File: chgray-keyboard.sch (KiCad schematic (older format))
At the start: 1 part, among them U1 Teensy2.0_(C)

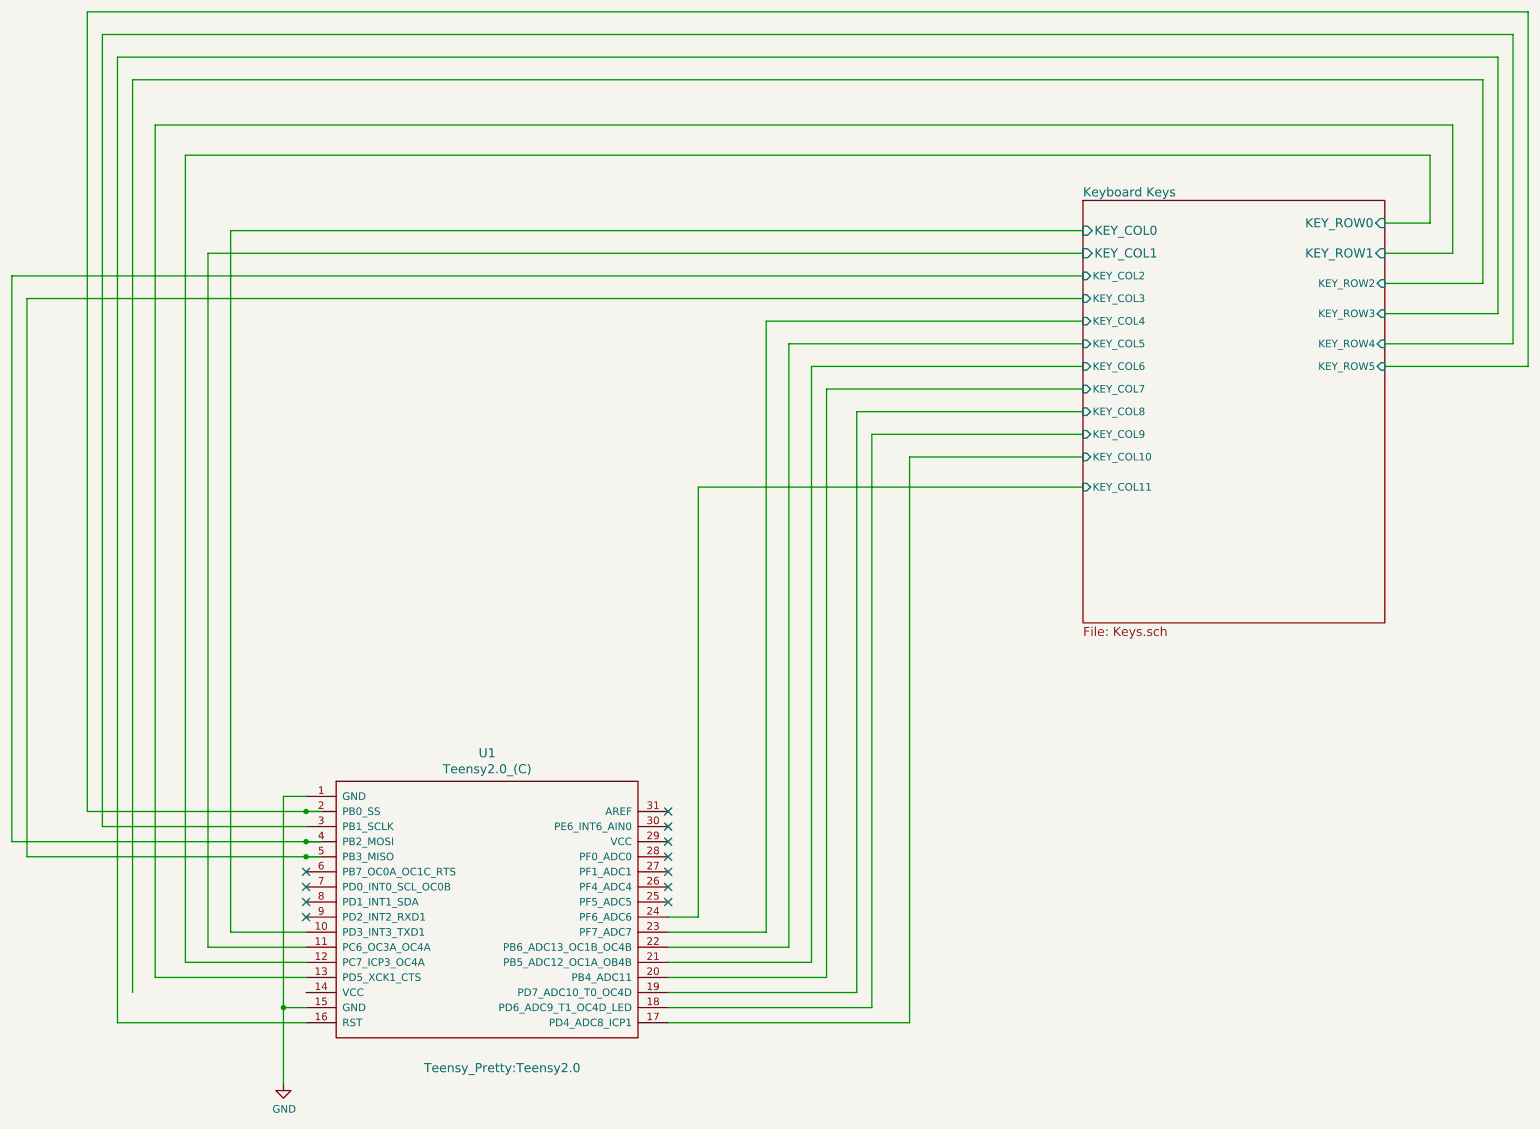
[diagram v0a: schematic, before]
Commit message: working on rgb
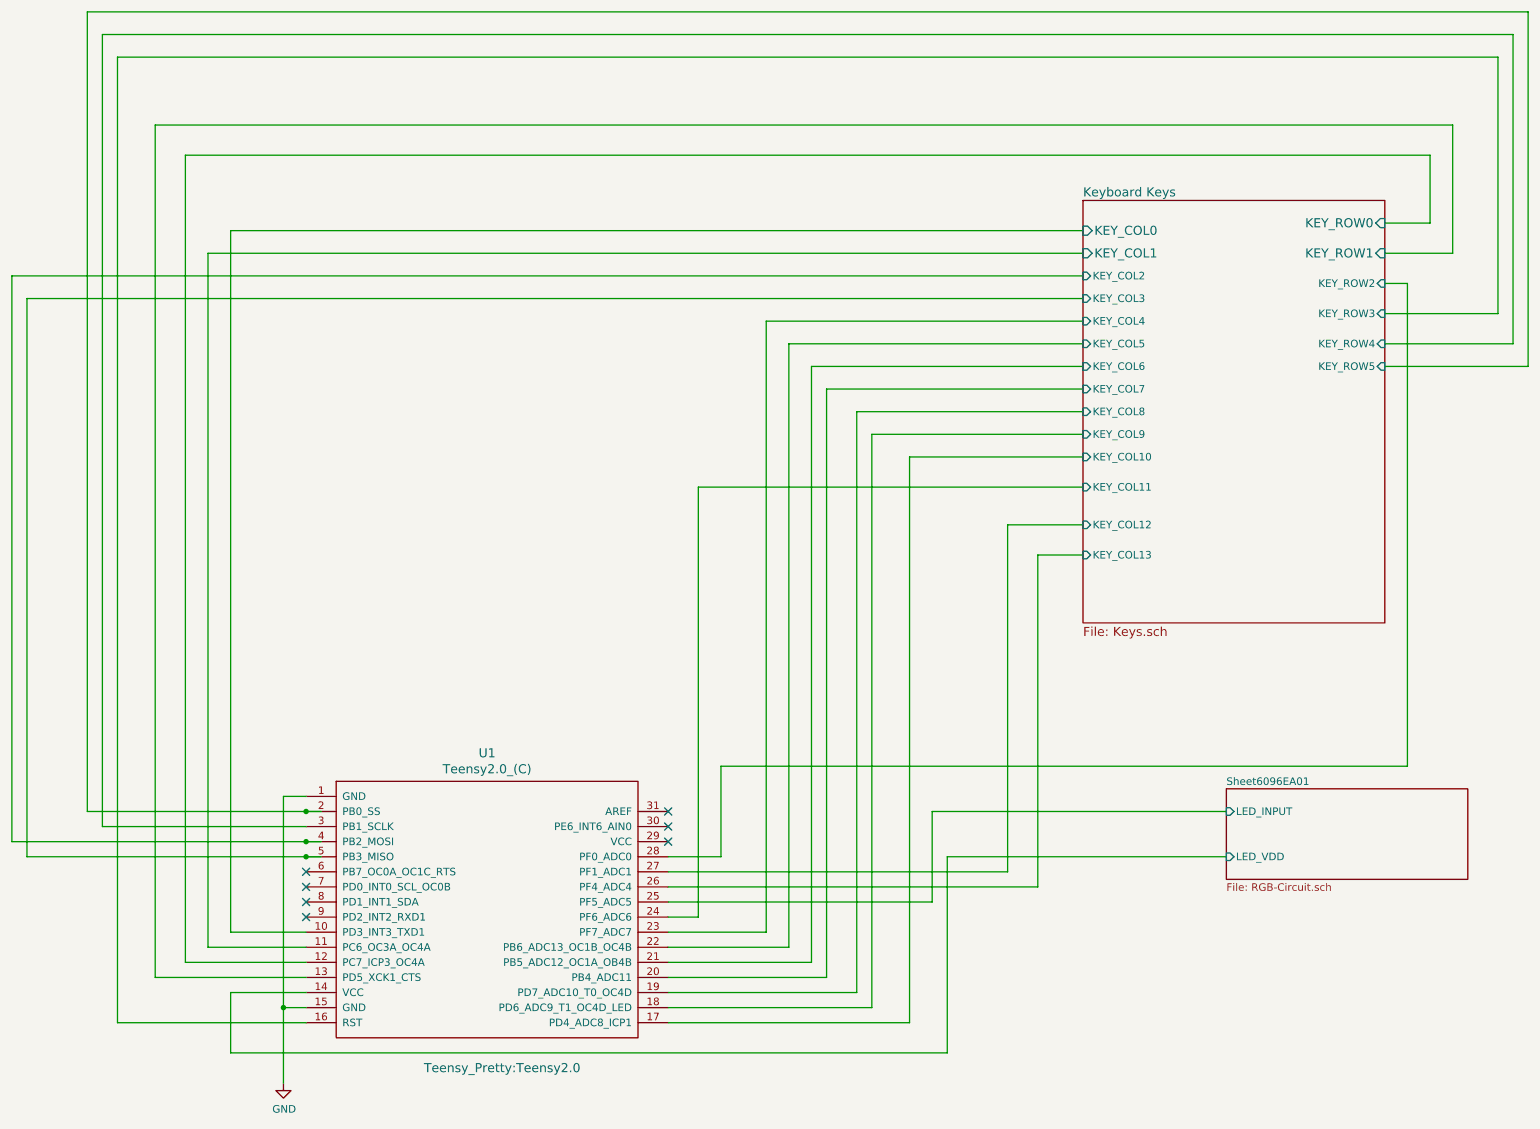
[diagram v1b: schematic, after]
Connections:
- wire segments 72 -> 87
- no-connect marks 11 -> 7
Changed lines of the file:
@@
 $Descr A 11000 8500
 encoding utf-8
-Sheet 1 2
+Sheet 1 3
 Title ""
 Date ""
@@
 F18 "KEY_COL10" I L 7300 3500 50
 F19 "KEY_COL11" I L 7300 3700 50
+F20 "KEY_COL12" I L 7300 3950 50
+F21 "KEY_COL13" I L 7300 4150 50
 $EndSheet
 Wire Wire Line
@@
 Wire Wire Line
 	1500 2150 7300 2150
-Wire Wire Line
-	9950 2350 9950 1000
-Wire Wire Line
-	9950 1000 1000 1000
 Wire Wire Line
 	10050 2550 10050 850
@@
 	900  850  900  7250
 Wire Wire Line
-	1000 1000 1000 7050
-Wire Wire Line
 	1150 6950 2150 6950
 Wire Wire Line
@@
 NoConn ~ 4550 5950
 NoConn ~ 4550 6050
-NoConn ~ 4550 6150
-NoConn ~ 4550 6250
-NoConn ~ 4550 6350
-NoConn ~ 4550 6450
 NoConn ~ 2150 6250
 NoConn ~ 2150 6350
@@
 	9300 2150 9750 2150
 Wire Wire Line
-	9300 2350 9950 2350
-Wire Wire Line
 	9300 2550 10050 2550
 Wire Wire Line
@@
 Wire Wire Line
 	9300 2900 10250 2900
+$Sheet
+S 8250 5700 1600 600
+U 6096EA02
+F0 "Sheet6096EA01" 50
+F1 "RGB-Circuit.sch" 50
+F2 "LED_INPUT" I L 8250 5850 50
+F3 "LED_VDD" I L 8250 6150 50
+$EndSheet
+Wire Wire Line
+	8250 5850 6300 5850
+Wire Wire Line
+	6300 5850 6300 6450
+Wire Wire Line
+	6300 6450 4550 6450
+Wire Wire Line
+	8250 6150 6400 6150
+Wire Wire Line
+	6400 6150 6400 7450
+Wire Wire Line
+	6400 7450 1650 7450
+Wire Wire Line
+	1650 7450 1650 7050
+Wire Wire Line
+	1650 7050 2150 7050
+Wire Wire Line
+	9300 2350 9450 2350
+Wire Wire Line
+	9450 2350 9450 5550
+Wire Wire Line
+	9450 5550 4900 5550
+Wire Wire Line
+	4900 5550 4900 6150
+Wire Wire Line
+	4900 6150 4550 6150
+Wire Wire Line
+	4550 6250 6800 6250
+Wire Wire Line
+	6800 6250 6800 3950
+Wire Wire Line
+	6800 3950 7300 3950
+Wire Wire Line
+	7300 4150 7000 4150
+Wire Wire Line
+	7000 4150 7000 6350
+Wire Wire Line
+	7000 6350 4550 6350
 $EndSCHEMATC
